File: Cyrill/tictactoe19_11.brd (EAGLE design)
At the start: 70.8 x 69.8 mm, 18 parts, among them IC1 PCF8574P, U1 ATMEGA328P_PDIP

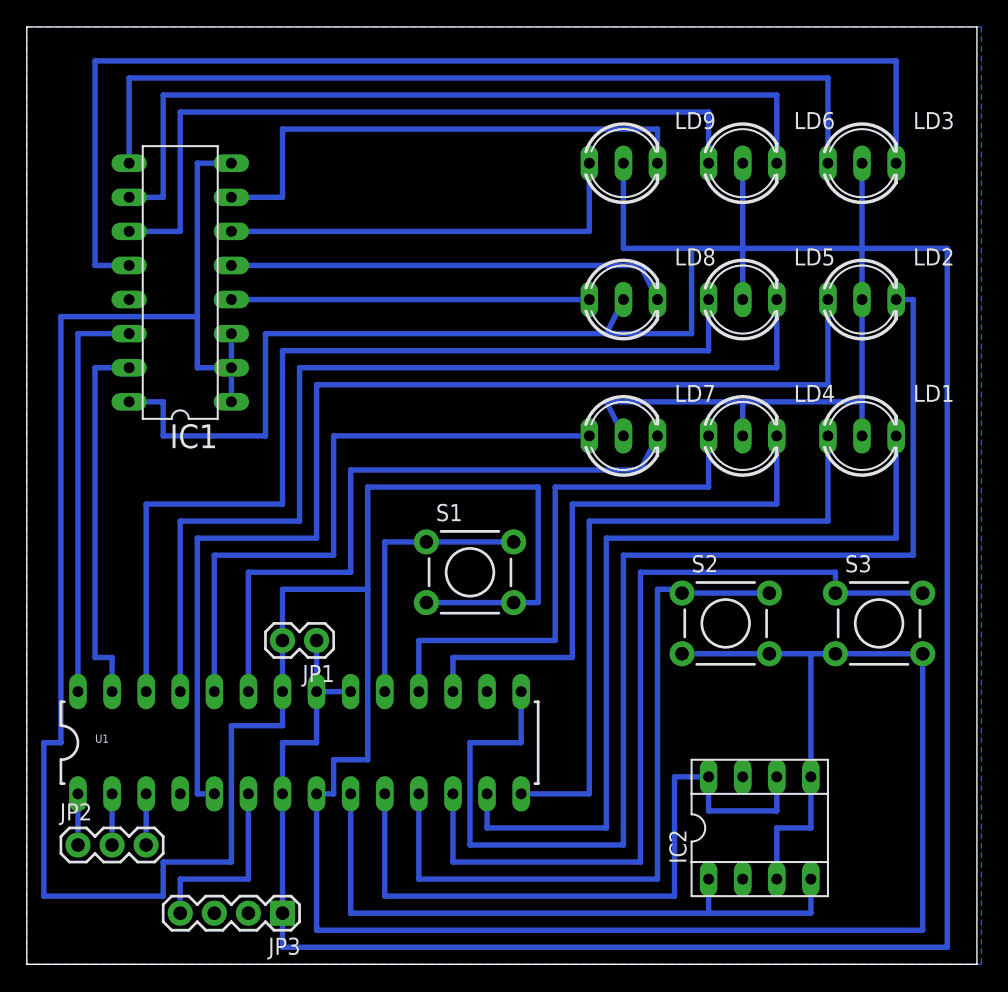
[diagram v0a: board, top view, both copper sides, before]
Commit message: final2
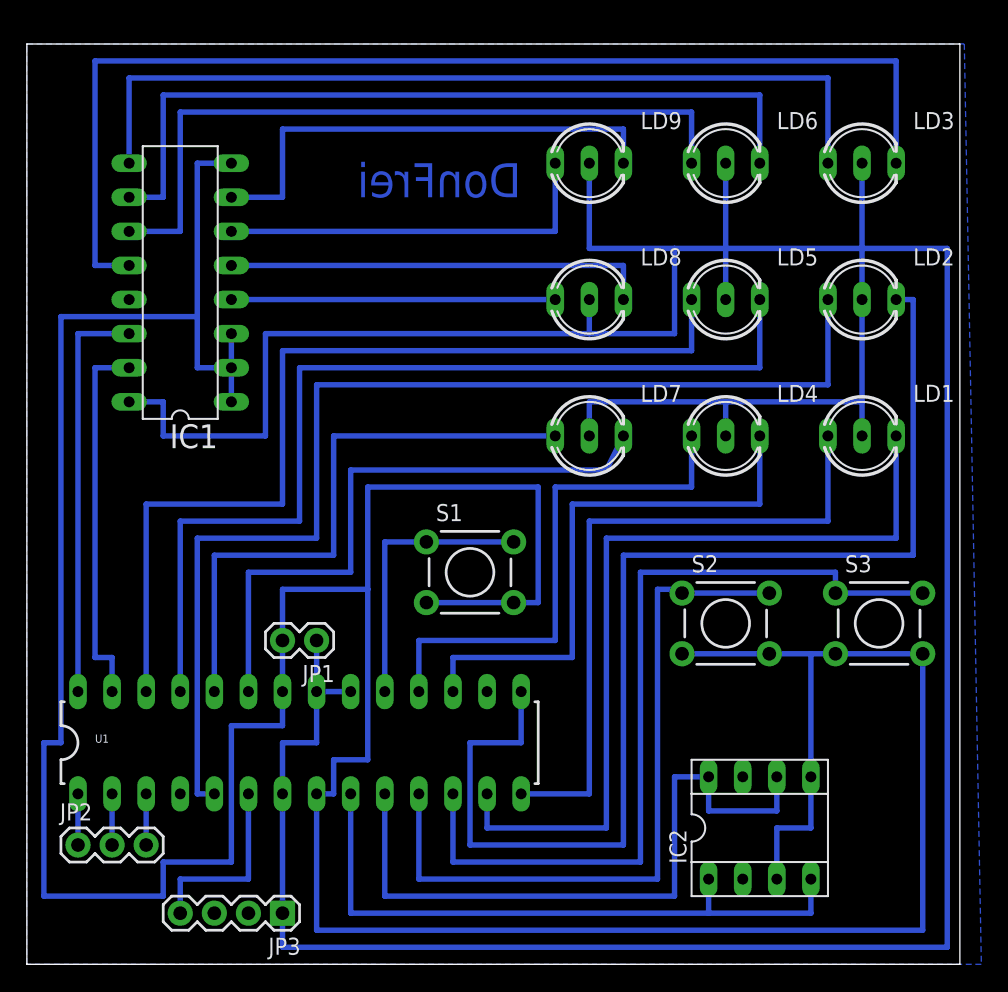
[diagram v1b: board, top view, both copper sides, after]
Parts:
- moved LD7 2.54 mm to (44.5, 35.6)
- moved LD8 2.54 mm to (44.5, 45.7)
- moved LD9 2.54 mm to (44.5, 55.9)
- moved LD4 1.27 mm to (54.6, 35.6)
- moved LD5 1.27 mm to (54.6, 45.7)
- moved LD6 1.27 mm to (54.6, 55.9)
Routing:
- net N$27: track 26.7 -> 24.1 mm
- net N$26: track 31.8 -> 29.2 mm
- net N$25: track 39.4 -> 36.8 mm
- net N$18: track 47.0 -> 44.4 mm
- net N$15: track 48.6 -> 46.0 mm
- net VCC: track 276.2 -> 278.1 mm
- net N$28: track 33.3 -> 31.8 mm
- net N$29: track 71.1 -> 69.8 mm
- net N$16: track 43.2 -> 41.9 mm
- net N$22: track 55.9 -> 54.6 mm
- net N$31: track 73.7 -> 72.4 mm
- net N$23: track 61.0 -> 59.7 mm
- net N$17: track 40.6 -> 39.4 mm
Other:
- board size 70.8 x 69.8 mm -> 69.5 x 68.6 mm
- board text added: "DonFrei"
